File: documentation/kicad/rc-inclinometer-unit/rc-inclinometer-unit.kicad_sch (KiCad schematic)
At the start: 1 part

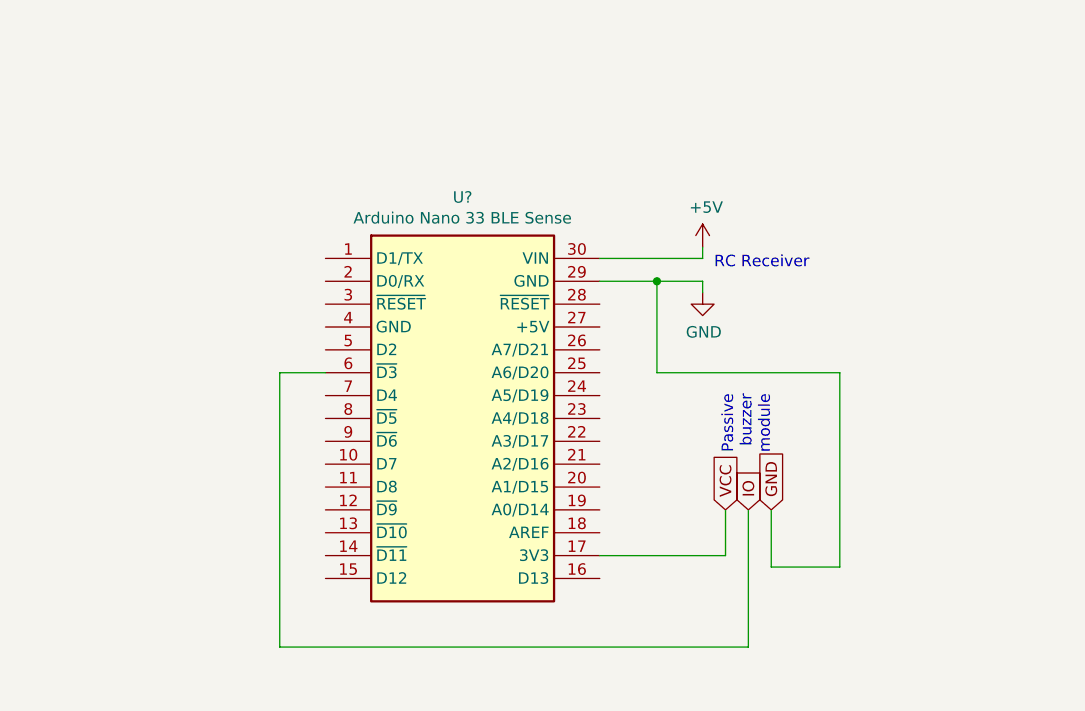
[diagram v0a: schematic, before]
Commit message: kicad schema update
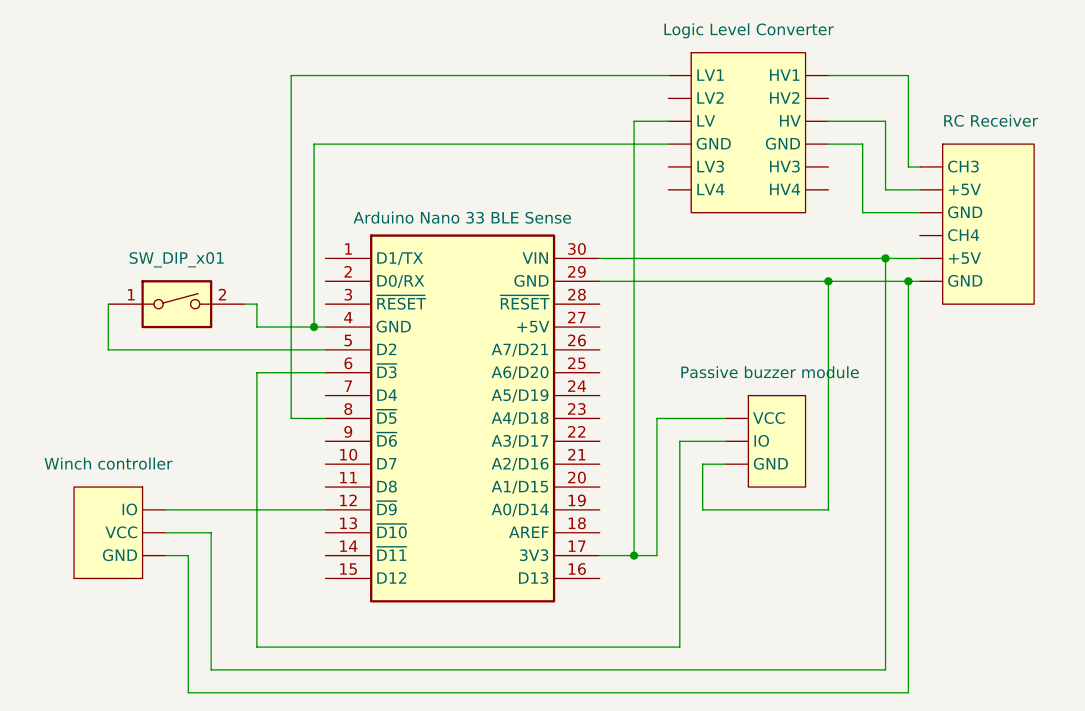
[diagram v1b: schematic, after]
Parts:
- added SW?: SW_DIP_x01, symbol Switch:SW_DIP_x01
- added U?: Winch controller, symbol rc-inclinometer-unit-custom-library:Winch controller
- added U?: Logic Level Converter, symbol rc-inclinometer-unit-custom-library:Logic Level Converter
- added U?: Passive buzzer module, symbol rc-inclinometer-unit-custom-library:Passive buzzer module
- added U?: RC Receiver, symbol rc-inclinometer-unit-custom-library:RC Receiver
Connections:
- net at U?.12 (~{D9}): now also U?. (VCC)
- net at U?.4 (GND): now also SW?.2, U?. (LV4)
- net at U?.5 (D2): now also SW?.1
- net at U?.8 (~{D5}): now also U?. (LV4)
- net +5V: no longer names the net of U?.30 (VIN)
- net +5V: now also U?. (GND), U?. (VCC)
- net GND: no longer names the net of U?.29 (GND)
- net GND: now also U?. (GND), U?. (VCC), U?. (VCC)
- net IO: no longer names the net of U?.6 (~{D3})
- net IO: now also U?. (VCC)
- net VCC: no longer names the net of U?.17 (3V3)
- net VCC: now also U?. (LV4), U?. (VCC)
- new net: U?. (GND), U?. (LV4) (x3)
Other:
- note removed: "Passive buzzer module"
- note removed: "RC Receiver"
